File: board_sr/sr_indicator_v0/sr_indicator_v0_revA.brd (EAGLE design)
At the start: 44 x 45 mm, 31 parts, among them IC1 ULN2004AD, IC2 ULN2004AD

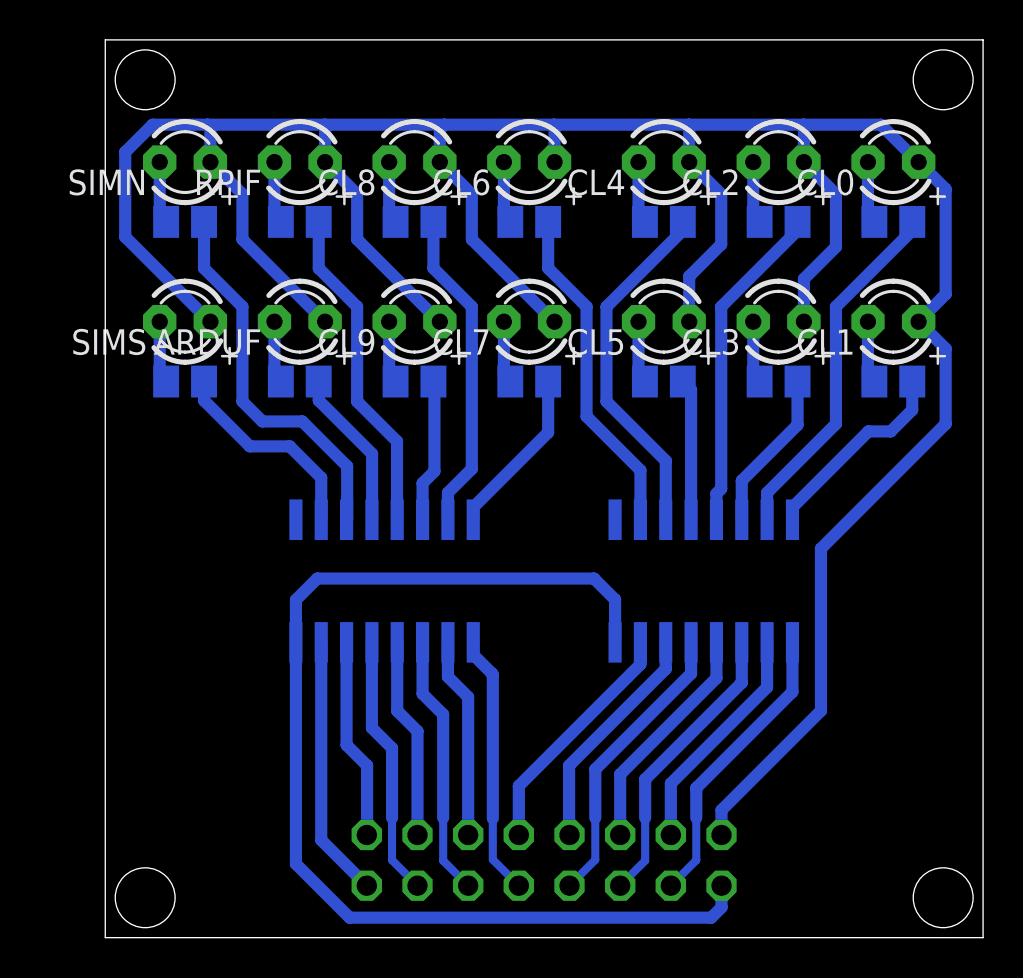
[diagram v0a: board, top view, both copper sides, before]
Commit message: Update casing
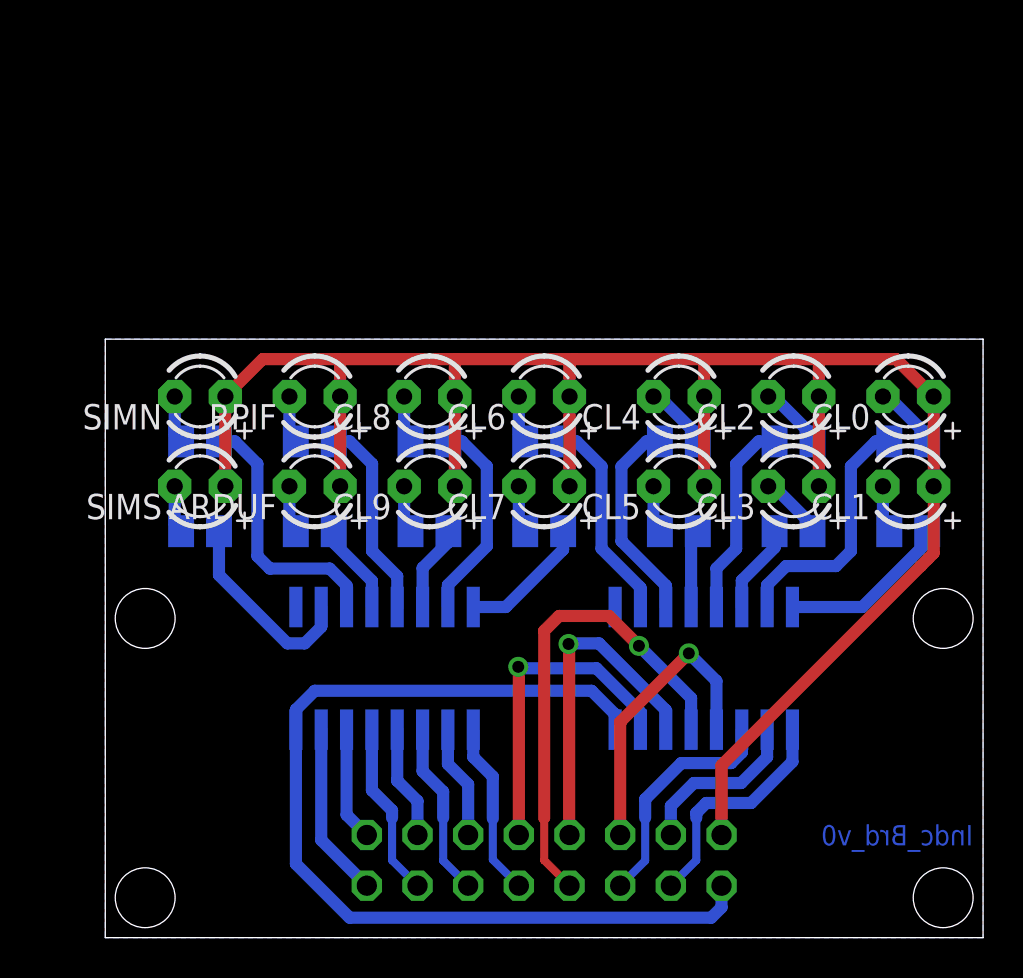
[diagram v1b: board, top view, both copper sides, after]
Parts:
- moved CL0 11.8 mm to (40.2, 27.1)
- moved CL2 11.8 mm to (34.5, 27.1)
- moved CL4 11.8 mm to (28.8, 27.1)
- moved CL6 11.8 mm to (22.0, 27.1)
- moved CL8 11.8 mm to (16.2, 27.1)
- moved RPIF 11.8 mm to (10.5, 27.1)
- moved SIMN 11.8 mm to (4.75, 27.1)
- moved R11 11.0 mm to (34.5, 24.9), turned to 180 degrees
- moved R13 11.0 mm to (28.8, 24.9), turned to 180 degrees
- moved R14 11.0 mm to (22.0, 24.9)
- moved R2 11.0 mm to (16.2, 24.9)
- moved R4 11.0 mm to (10.5, 24.9)
- moved R6 11.0 mm to (4.75, 24.9)
- moved R9 11.0 mm to (40.2, 24.9), turned to 180 degrees
- moved ARDUF 8.28 mm to (10.5, 22.6)
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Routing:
- net +5V: track 152.7 -> 100.1 mm
- net CTRL_LED5: track 14.7 -> 24.3 mm, vias 0 -> 1
- net N$20: track 17.7 -> 10.4 mm
- net GND: track 56.0 -> 49.1 mm
- net N$18: track 16.6 -> 9.98 mm
- net N$21: track 16.8 -> 10.3 mm
- net N$4: track 16.6 -> 10.1 mm
- net N$2: track 16.2 -> 10.3 mm
- net N$6: track 19.1 -> 13.2 mm
- net N$16: track 17.9 -> 12.7 mm
- net CTRL_LED4: track 11.7 -> 16.8 mm, vias 0 -> 1
- net SIM_NETLIGHT: track 10.1 -> 5.70 mm
- net CTRL_LED7: track 13.1 -> 8.77 mm
- net ARDU_FLASH: track 13.1 -> 8.77 mm
- net SIM_STATUS: track 13.1 -> 8.77 mm
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- added copper zone on layer 16, net GND
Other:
- board size 44 x 45 mm -> 44 x 30 mm
- board text added: "Indc_Brd_v0"

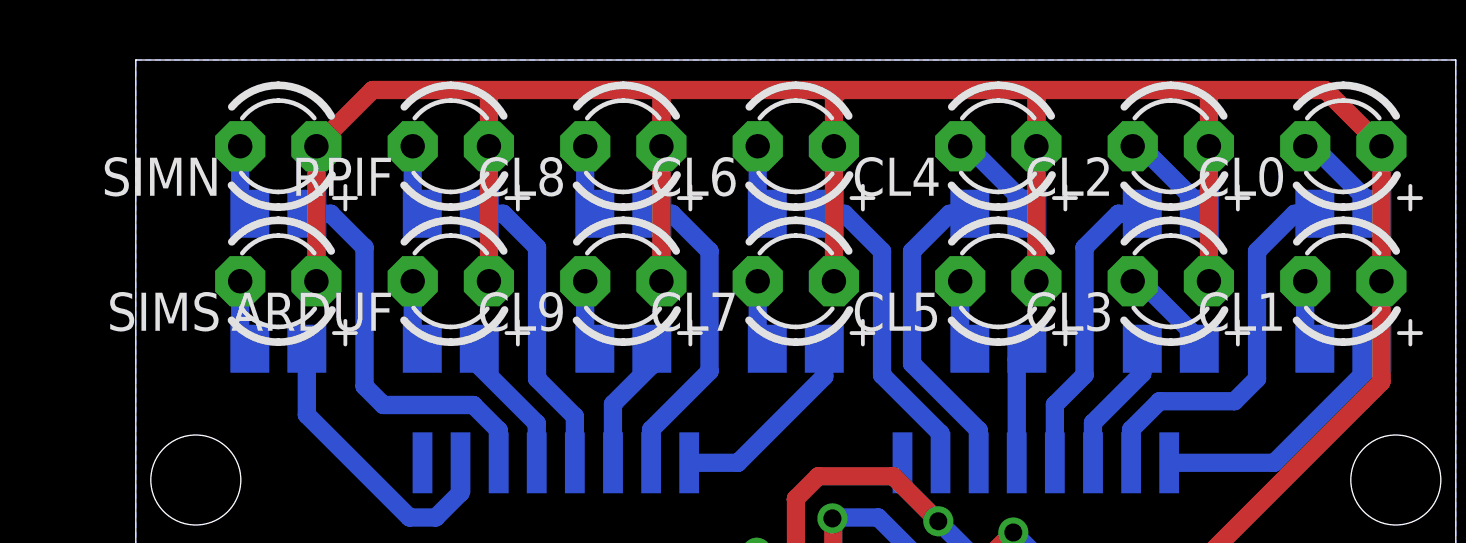
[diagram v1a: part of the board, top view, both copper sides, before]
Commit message: Publish sr_controller_v1_revC
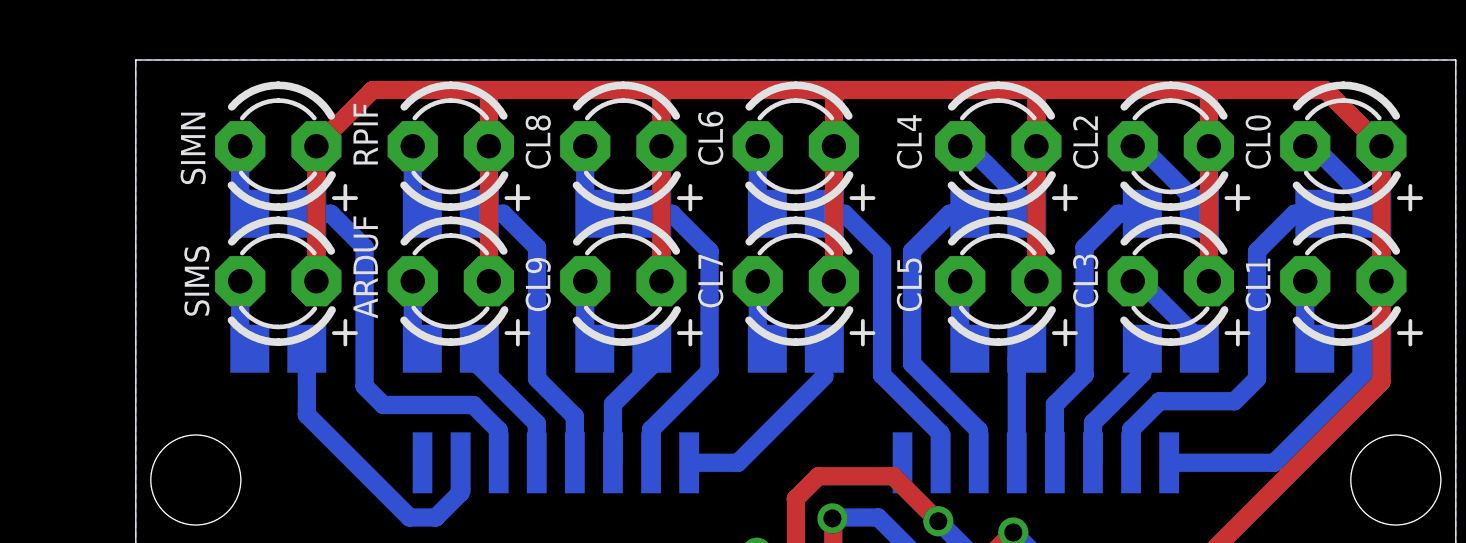
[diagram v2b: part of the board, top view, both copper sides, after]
